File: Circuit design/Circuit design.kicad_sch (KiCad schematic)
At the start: 6 parts, among them T1 ZMPT101B, U1 LM358, U2 TL431LP

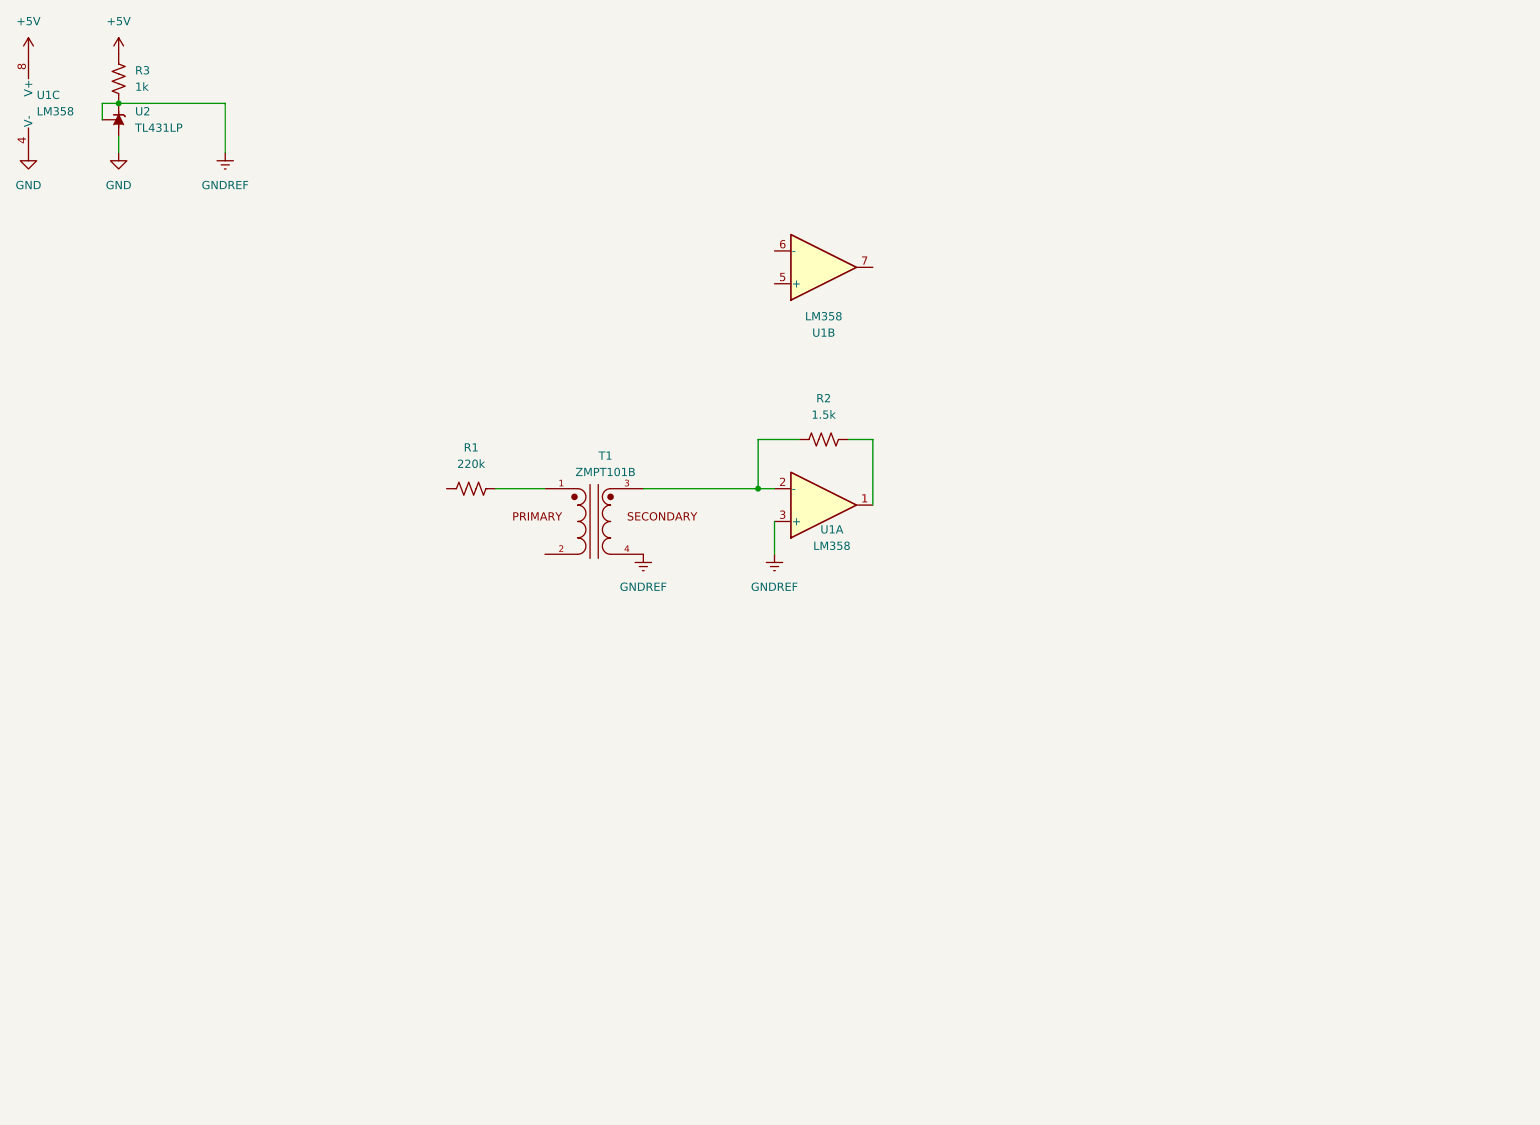
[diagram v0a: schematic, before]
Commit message: Updated Circuit Diagram
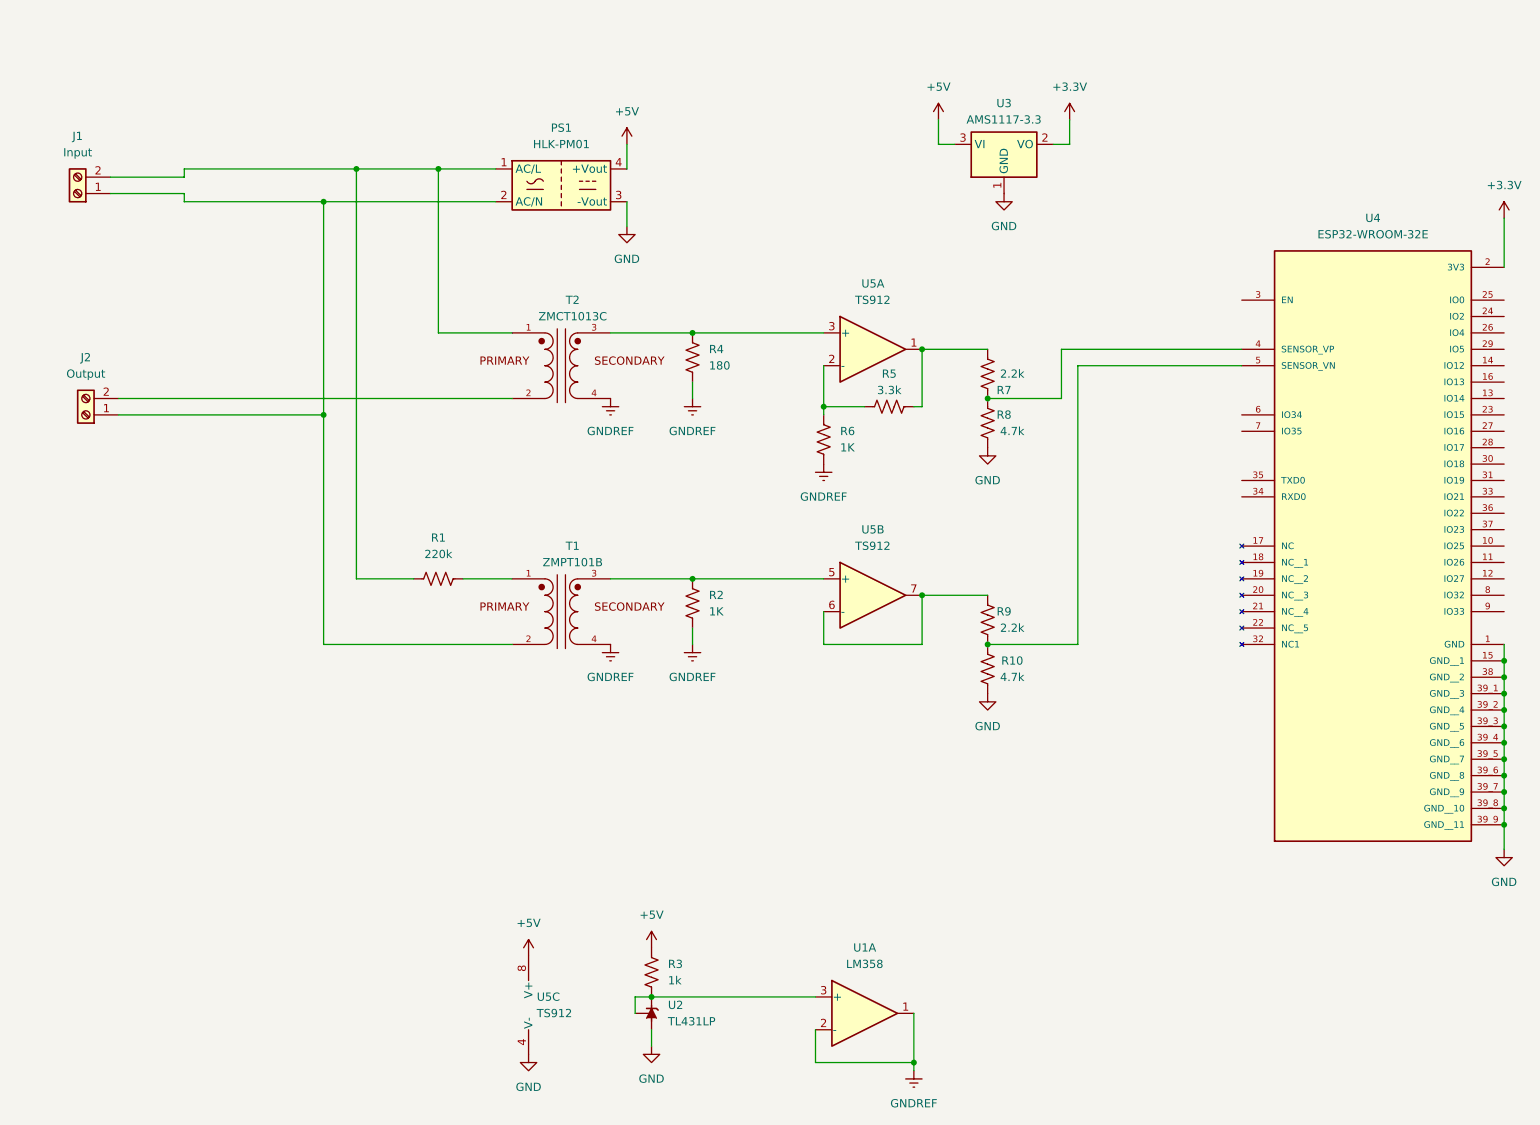
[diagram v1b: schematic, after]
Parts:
- removed unit 3 of U1
- removed unit 2 of U1
- added J1: Input, symbol Connector:Screw_Terminal_01x02
- added J2: Output, symbol Connector:Screw_Terminal_01x02
- added PS1: HLK-PM01, Converter_ACDC:Converter_ACDC_HiLink_HLK-PMxx, symbol Converter_ACDC:HLK-PM01
- added R10, R8: 4.7k, symbol Device:R_US
- added R4: 180, symbol Device:R_US
- added R5: 3.3k, symbol Device:R_US
- added R6: 1K, symbol Device:R_US
- added R7, R9: 2.2k, symbol Device:R_US
- added T2: ZMCT1013C, symbol ZMPT101B:ZMPT101B
- added U3: AMS1117-3.3, Package_TO_SOT_SMD:SOT-223-3_TabPin2, symbol Regulator_Linear:AMS1117-3.3
- added U4: ESP32-WROOM-32E, ESP32-WROOM-32E__16MB_:XCVR_ESP32-WROOM-32E__16MB_, symbol ESP32-WROOM-32E_:ESP32-WROOM-32E
- added U5: TS912, symbol Amplifier_Operational:TS912
- R2: value 1.5k -> 1K
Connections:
- net +5V: now also PS1.4 (+Vout), U3.3 (VI), U5.8 (V+)
- net GND: now also PS1.3 (-Vout), R10.2, R8.2, U3.1 (GND), U4.1 (GND), U4.15 (GND__1), U4.38 (GND__2), U4.39_1 (GND__3), U4.39_2 (GND__4), U4.39_3 (GND__5), U4.39_4 (GND__6), U4.39_5 (GND__7), U4.39_6 (GND__8), U4.39_7 (GND__9), U4.39_8 (GND__10), U4.39_9 (GND__11), U5.4 (V-)
- net GNDREF: now also R2.1, U1.1, U1.2 (-), R4.1, R6.1, T2.4; no longer R3.2, U1.3 (+), U2.1 (REF), U2.3 (K)
- net at R2.2: now also T1.3, U5.5 (+); no longer U1.1
- net at R1.1: now also J1.2 (Pin_2), PS1.1 (AC/L), T2.1
- net at T1.2: now also J1.1 (Pin_1), J2.1 (Pin_1), PS1.2 (AC/N)
- new net: R5.2, R7.1, U5.1
- new net: R5.1, R6.2, U5.2 (-)
- new net: R4.2, T2.3, U5.3 (+)
- new net: R7.2, R8.1, U4.4 (SENSOR_VP)
- new net: R10.1, R9.2, U4.5 (SENSOR_VN)
- new net: R9.1, U5.6 (-), U5.7
- new net: J2.2 (Pin_2), T2.2
- new net: R3.2, U1.3 (+), U2.1 (REF), U2.3 (K)
- new net +3.3V: U3.2 (VO), U4.2 (3V3)
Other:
- moved on the sheet: R1, R2, R3, T1, U2
